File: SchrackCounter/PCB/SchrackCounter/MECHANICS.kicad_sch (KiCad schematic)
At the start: 25 parts, among them J3 Conn_01x02_Pin, J4 Conn_01x02_Pin, J5 MEM2067-02-180-00-A_REVB, M1 Fan_CPU_4pin, SW1 SW_Push, SW2 SW_Push, SW3 SW_Push, SW4 SW_Push, SW5 SW_Push, SW6 RotaryEncoder_Switch

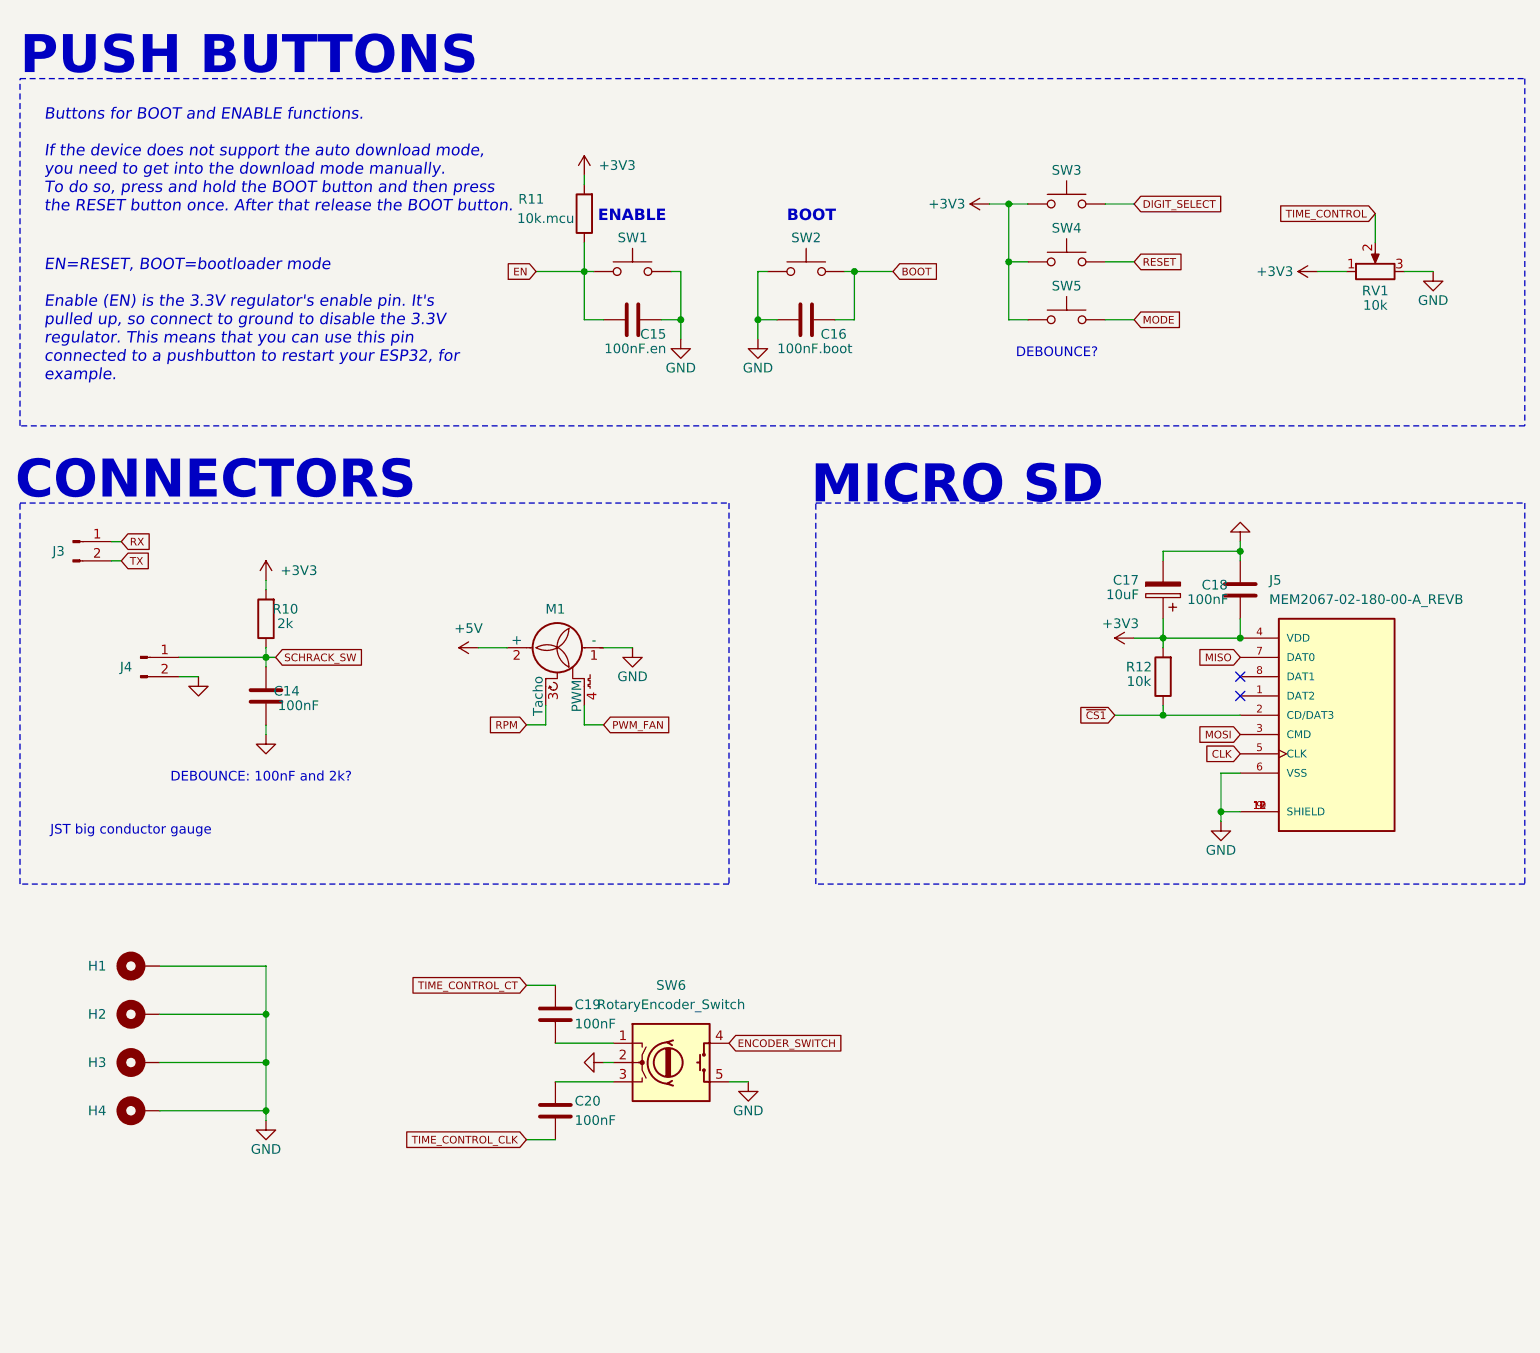
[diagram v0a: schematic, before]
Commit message: schematic and board update
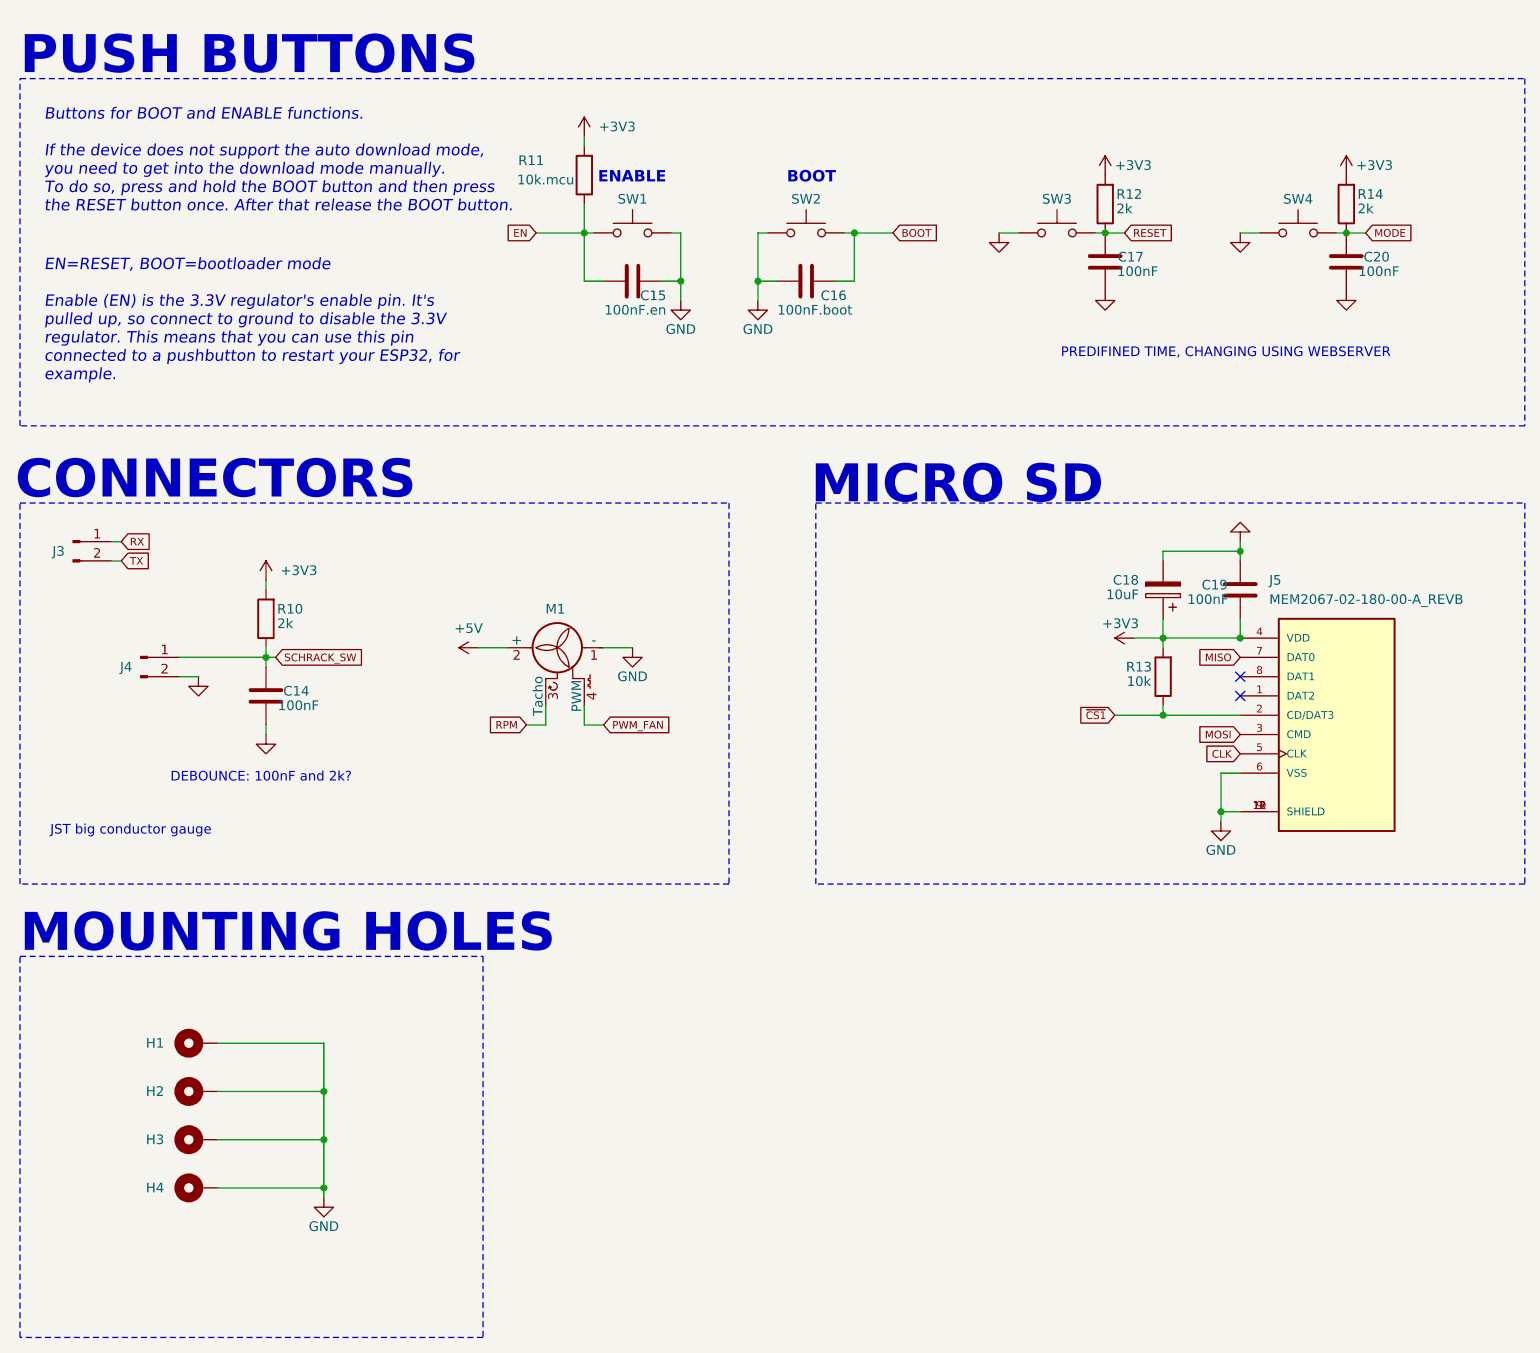
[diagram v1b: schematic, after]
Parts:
- removed C19: 100nF, Capacitor_SMD:C_0805_2012Metric_Pad1.18x1.45mm_HandSolder, symbol Device:C
- removed RV1: 10k, Connector_JST:JST_XH_B3B-XH-A_1x03_P2.50mm_Vertical, symbol Device:R_Potentiometer
- removed SW3: SW_Push, Connector_JST:JST_XH_B2B-XH-A_1x02_P2.50mm_Vertical, symbol Switch:SW_Push
- removed SW5: SW_Push, Button_Switch_SMD:SW_SPST_EVQPE1, symbol Switch:SW_Push
- removed SW6: RotaryEncoder_Switch, Connector_JST:JST_XH_B4B-XH-A_1x04_P2.50mm_Vertical, symbol SchrackThingy_library:RotaryEncoder_Switch
- added C17: 100nF, Capacitor_SMD:C_0805_2012Metric_Pad1.18x1.45mm_HandSolder, symbol Device:C
- added R12, R14: 2k, Resistor_SMD:R_0805_2012Metric_Pad1.20x1.40mm_HandSolder, symbol Device:R
- added SW4: SW_Push, Connector_JST:JST_XH_B2B-XH-A_1x02_P2.50mm_Vertical, symbol Switch:SW_Push
- C20: LCSC C49678 -> (none)
- renumbered C17 to C18, C18 to C19, R12 to R13, SW4 to SW3
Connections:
- net TIME_CONTROL_CLK is gone; now on net MODE: C20.2
- net +3V3: now also R12.2, R14.2; no longer SW3.1
- net GND: now also C20.1, SW3.1, C17.1, SW4.1
- net MODE: now also R14.1, SW4.2
- net RESET: now also C17.2, R12.1
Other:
- note added: "MOUNTING HOLES"
- note added: "PREDIFINED TIME, CHANGING USING WEBSERVER"
- note removed: "DEBOUNCE?"
- moved on the sheet: C15, C16, H1, H2, H3, H4, R11, SW1, SW2, SW3
